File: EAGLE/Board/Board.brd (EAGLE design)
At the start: 50 x 50 mm, 19 parts

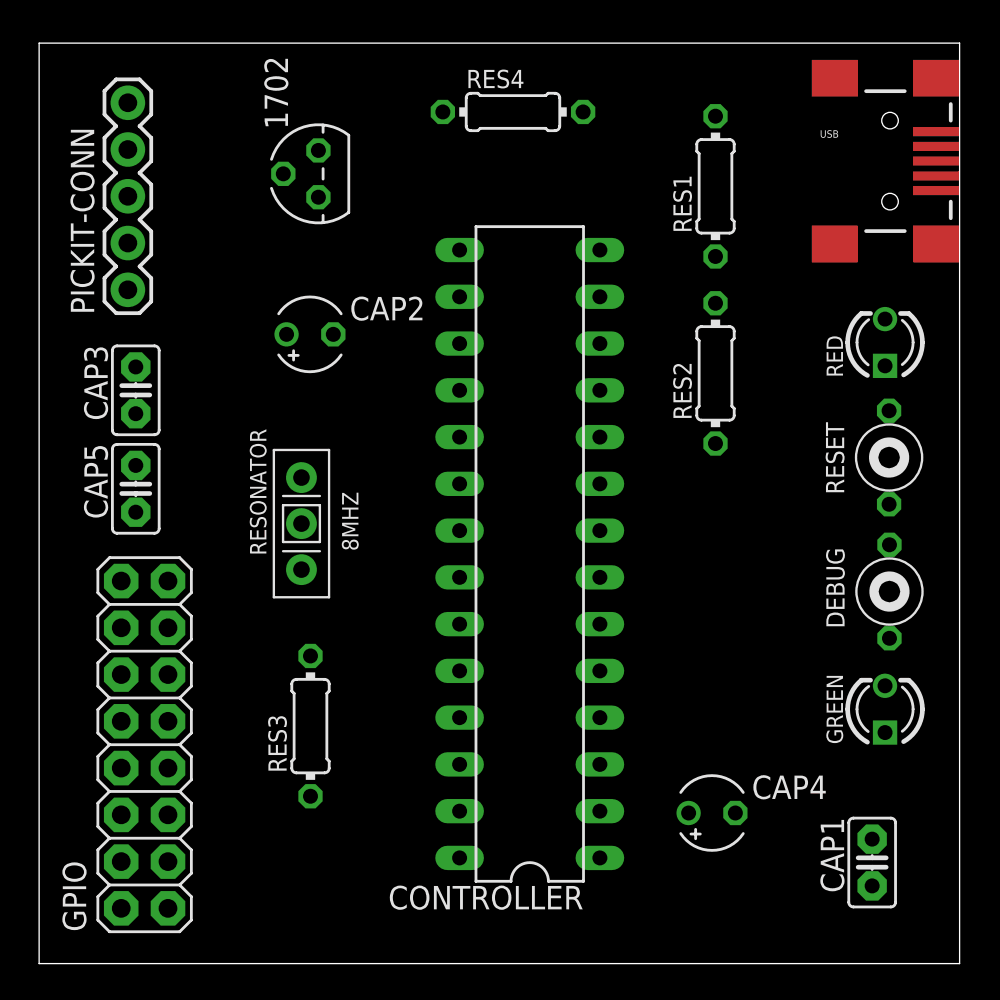
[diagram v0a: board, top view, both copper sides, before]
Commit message: board
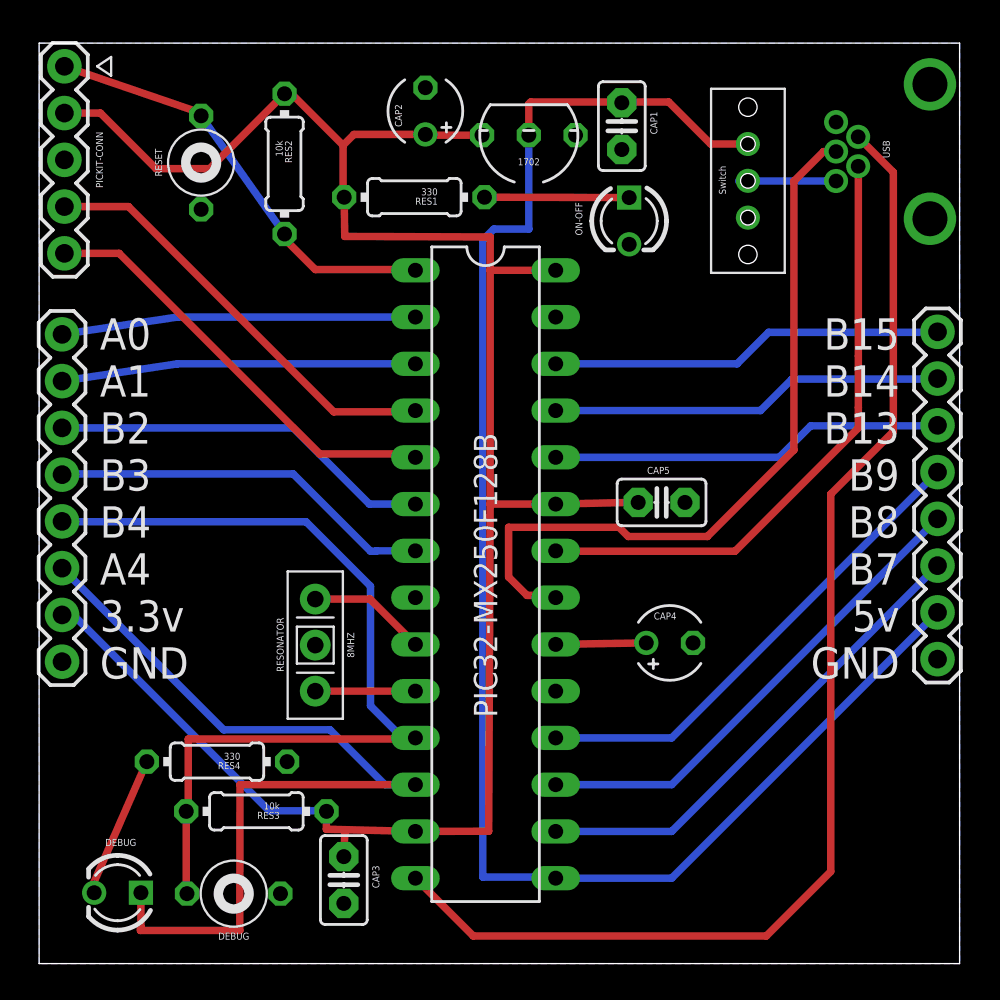
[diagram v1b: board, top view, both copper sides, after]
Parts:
- removed CONTROLLER: PIC32-MX250F128B, 433:DIL28-3
- removed GPIO: (no value), 433:2X8
- added GPIO1, GPIO2: (no value), 433:1X08_ROUND
- added PIC32-MX250F128B: PIC32-MX250F128B, 433:DIL28-3
- added U$1: SWITCH, 433:SWITCH
- 1702: value (none) -> REGULATORLMLZ
- RESONATOR: device 433:X3-2.5-8X3X5.5MM -> 433:OSCILATOR-CRYSTAL
- USB: value (none) -> USB-MINIB; device 433:USB-MINIB -> 433:USB-MB-H
- moved GREEN 42.9 mm to (4.26, 3.85), turned to 180 degrees
- moved CAP1 42.2 mm to (31.6, 45.5), turned to 270 degrees
- moved RESET 40.7 mm to (8.80, 43.5)
- moved DEBUG 39.2 mm to (10.6, 3.80), turned to 180 degrees
- moved RES4 38.8 mm to (9.66, 11.0), turned to 180 degrees
- moved CAP3 28.9 mm to (16.6, 4.54), turned to 270 degrees
- moved CAP5 28.6 mm to (33.8, 25.1), turned to 0 degrees
- moved RES2 26.0 mm to (13.3, 43.4), turned to 270 degrees
- moved RES1 16.4 mm to (20.4, 41.6), turned to 180 degrees
- moved RED 15.4 mm to (32.0, 40.3), turned to 270 degrees
- moved CAP2 13.7 mm to (21.0, 46.3), turned to 90 degrees
- moved PICKIT-CONN 12.6 mm to (1.37, 48.7), turned to 270 degrees
- moved 1702 11.6 mm to (26.6, 45.0), turned to 180 degrees
- moved CAP4 9.52 mm to (34.2, 17.4)
- moved RESONATOR 6.64 mm to (15.0, 17.3)
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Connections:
- new net N$8: U$1.IN, USB.VBUS
- net +3.3: now also GPIO1.7, PIC32-MX250F128B.13, PIC32-MX250F128B.23, PIC32-MX250F128B.28; no longer CONTROLLER.13, CONTROLLER.23, CONTROLLER.28, GPIO.2
- net +5: now also GPIO2.2, PIC32-MX250F128B.15, U$1.OA; no longer CONTROLLER.15, GPIO.4, USB.VBUS
- net GND: now also GPIO1.8, GPIO2.1, PIC32-MX250F128B.19, PIC32-MX250F128B.27, PIC32-MX250F128B.8; no longer CONTROLLER.19, CONTROLLER.27, CONTROLLER.8, GPIO.1, GPIO.3
- net N$1: now also PIC32-MX250F128B.10; no longer CONTROLLER.10
- net N$2: now also PIC32-MX250F128B.9; no longer CONTROLLER.9
- net N$4: now also PIC32-MX250F128B.4; no longer CONTROLLER.4
- net N$5: now also PIC32-MX250F128B.20; no longer CONTROLLER.20
- net N$7: now also PIC32-MX250F128B.1; no longer CONTROLLER.1
- net N$9: now also PIC32-MX250F128B.5; no longer CONTROLLER.5
- net RA0: now also GPIO1.1, PIC32-MX250F128B.2; no longer CONTROLLER.2, GPIO.5
- net RA1: now also GPIO1.2, PIC32-MX250F128B.3; no longer CONTROLLER.3, GPIO.7
- net RA4: now also GPIO1.6, PIC32-MX250F128B.12; no longer CONTROLLER.12, GPIO.15
- net RB13: now also GPIO2.6, PIC32-MX250F128B.24; no longer CONTROLLER.24, GPIO.10
- net RB14: now also GPIO2.7, PIC32-MX250F128B.25; no longer CONTROLLER.25, GPIO.8
- net RB15: now also GPIO2.8, PIC32-MX250F128B.26; no longer CONTROLLER.26, GPIO.6
- net RB2: now also GPIO1.3, PIC32-MX250F128B.6; no longer CONTROLLER.6, GPIO.9
- net RB3: now also GPIO1.4, PIC32-MX250F128B.7; no longer CONTROLLER.7, GPIO.11
- net RB4: now also GPIO1.5, PIC32-MX250F128B.11; no longer CONTROLLER.11, GPIO.13
- net RB7: now also GPIO2.3, PIC32-MX250F128B.16; no longer CONTROLLER.16, GPIO.16
- net RB8: now also GPIO2.4, PIC32-MX250F128B.17; no longer CONTROLLER.17, GPIO.14
- net RB9: now also GPIO2.5, PIC32-MX250F128B.18; no longer CONTROLLER.18, GPIO.12
- net USB-D+: now also PIC32-MX250F128B.21; no longer CONTROLLER.21
- net USB-D-: now also PIC32-MX250F128B.22; no longer CONTROLLER.22
- net USB-ID: now also PIC32-MX250F128B.14; no longer CONTROLLER.14
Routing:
- net +3.3: track 0.00 -> 114.0 mm
- net +5: track 0.00 -> 88.3 mm
- net USB-ID: track 0.00 -> 67.4 mm
- net RB4: track 0.00 -> 49.4 mm
- net RA4: track 0.00 -> 49.0 mm
- net USB-D+: track 0.00 -> 40.9 mm
- net USB-D-: track 0.00 -> 33.6 mm
- net RB9: track 0.00 -> 26.7 mm
- net RB8: track 0.00 -> 26.7 mm
- net RB7: track 0.00 -> 26.7 mm
- net N$7: track 0.00 -> 23.9 mm
- net N$4: track 0.00 -> 23.7 mm
- net N$9: track 0.00 -> 23.7 mm
- net RB15: track 0.00 -> 21.5 mm
- net RB14: track 0.00 -> 21.5 mm
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- added copper zone on layer 16, net GND
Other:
- board text added: "A0 A1 B2 B3 B4 A4 3.3v GND"
- board text added: "B15 B14 B13 B9 B8 B7 5v GND"
- board text added: "German Espinosa germanespinosa@gmail.com"
